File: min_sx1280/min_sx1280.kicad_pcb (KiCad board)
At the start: 2 copper layers, 20.5 x 17.4 mm, 15 parts, among them J1 Conn_01x04, SW1 SW_SPST, U1 ME6211C33, U2 ESP-01F, U3 LoRa1280

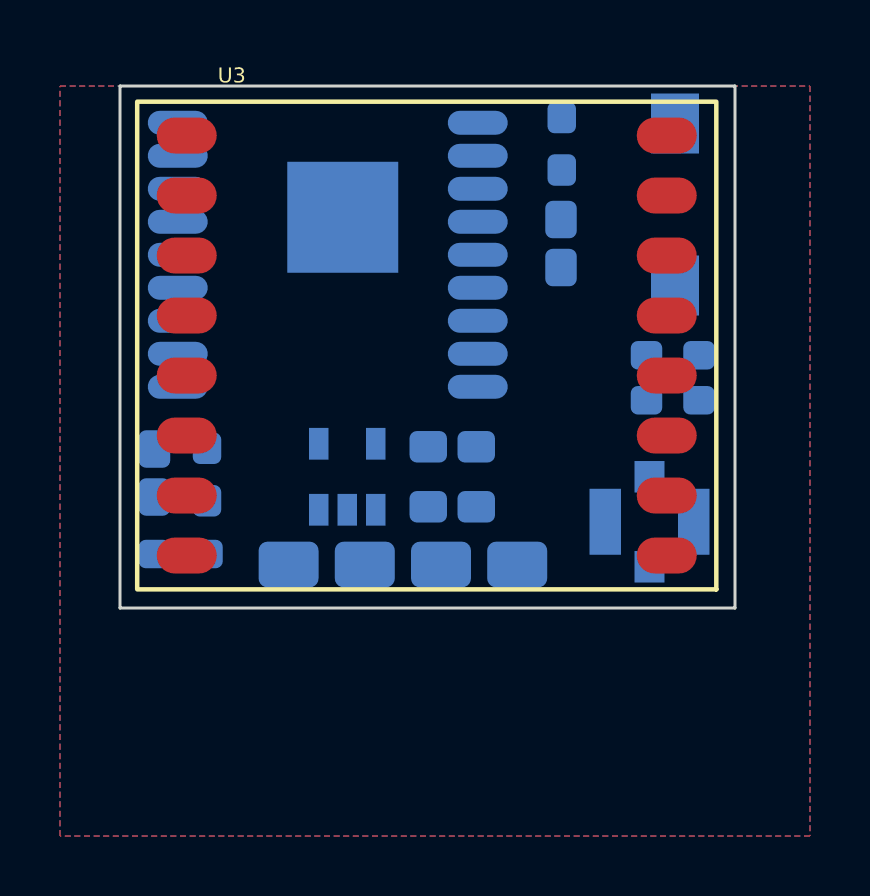
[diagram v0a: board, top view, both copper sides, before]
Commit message: Minimal RX ready to route
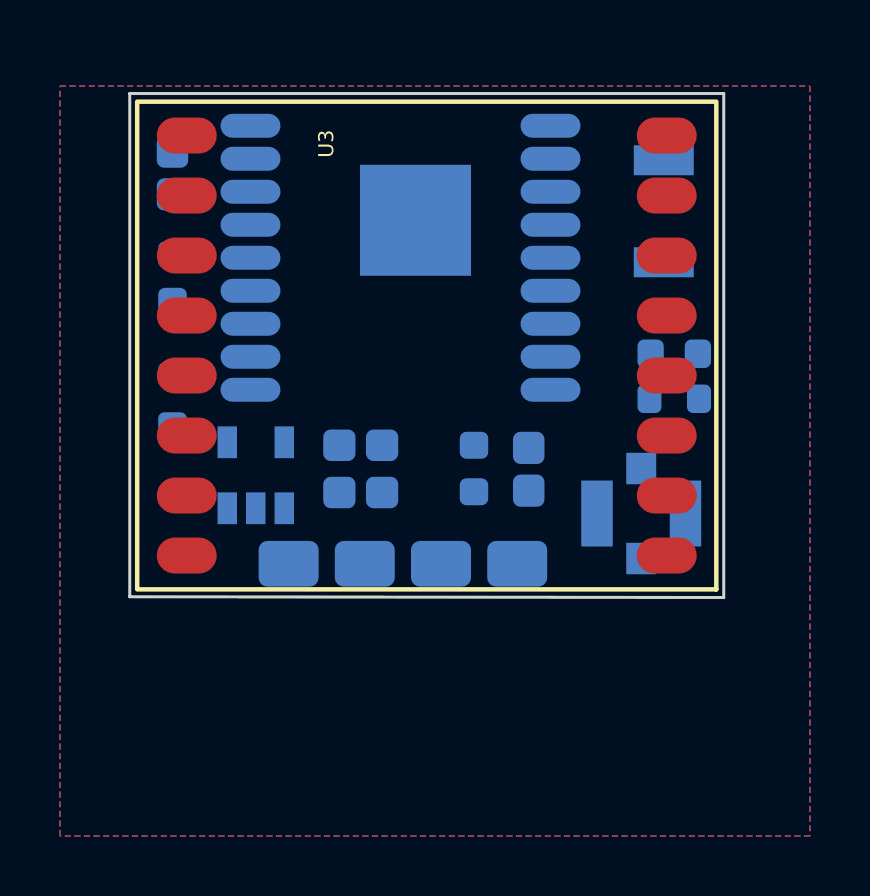
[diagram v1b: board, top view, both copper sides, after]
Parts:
- C1, C2, C5, C6: footprint Capacitor_Tantalum_SMD:CP_EIA-1608-08_AVX-J_Pad1.25x1.05mm_HandSolder -> Capacitor_Tantalum_SMD:CP_EIA-1608-08_AVX-J
- C3, C4: footprint Capacitor_SMD:C_0603_1608Metric_Pad1.05x0.95mm_HandSolder -> Capacitor_SMD:C_0603_1608Metric
- D1: footprint LED_SMD:LED_0603_1608Metric_Pad1.05x0.95mm_HandSolder -> LED_SMD:LED_0603_1608Metric
- R3, R4: footprint Resistor_SMD:R_0603_1608Metric_Pad1.05x0.95mm_HandSolder -> Resistor_SMD:R_0603_1608Metric
- SW1: footprint Button_Switch_SMD:SW_SPST_EVQPE1 -> ELRS_lib:SW_3x4x2
- moved C3 11.2 mm to (111.3, 140.2), turned to -90 degrees
- moved C6 10.0 mm to (101.2, 130.4)
- moved C5 7.60 mm to (113.1, 140.3)
- moved C4 6.65 mm to (101.2, 133.9)
- moved R3 5.16 mm to (101.2, 137.9), turned to -90 degrees
- moved C1 3.09 mm to (107.5, 141.1)
- moved C2 3.05 mm to (107.5, 139.5)
- moved U1 3.05 mm to (104.0, 140.5)
- moved U2 2.43 mm to (108.8, 133.2)
- moved SW1 0.44 mm to (117.6, 131.7)
- moved AE2 0.39 mm to (116.9, 141.8)
- moved D1 0.07 mm to (118.0, 136.4)
- moved R4 0.07 mm to (118.0, 137.9)
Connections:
- U2 pad 1: (no net) -> Net-(U2-Pad1)
- U2 pad 16: (no net) -> /RST
- U2 pad 3: (no net) -> Net-(U2-Pad3)
- U2 pad 4: (no net) -> /EN
- U3 pad 1: (no net) -> Net-(U3-Pad1)
- U3 pad 2: (no net) -> Net-(U3-Pad2)
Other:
- board size 20.5 x 17.4 mm -> 19.8 x 16.8 mm
